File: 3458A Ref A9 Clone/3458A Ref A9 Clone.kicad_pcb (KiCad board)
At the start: 4 copper layers, 50 x 42.5 mm, 44 parts, among them J400 Molex KK 254, J401 Molex KK 254, Q1 MMBF4392, Q401 BD139, U401 ADR/LTZ1000(A), U402 LT1013

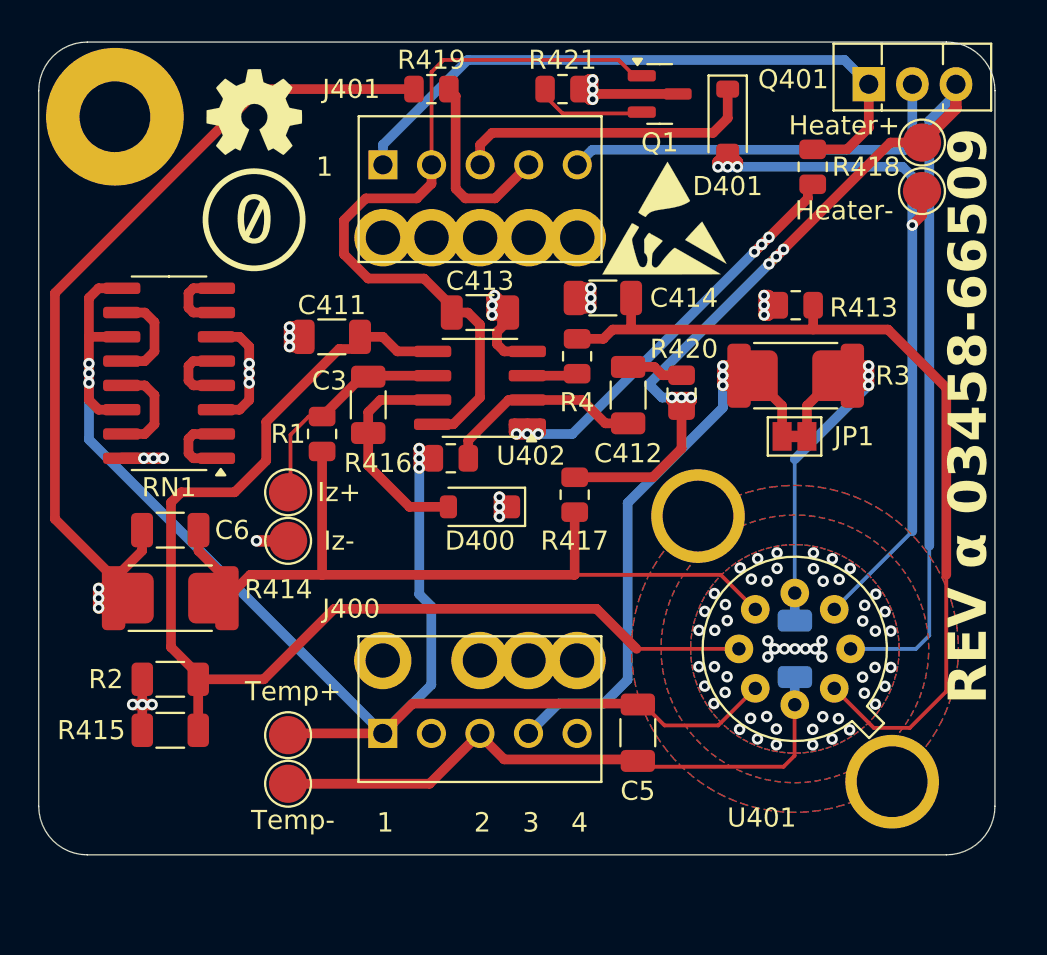
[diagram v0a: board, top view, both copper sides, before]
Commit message: Update to REV β
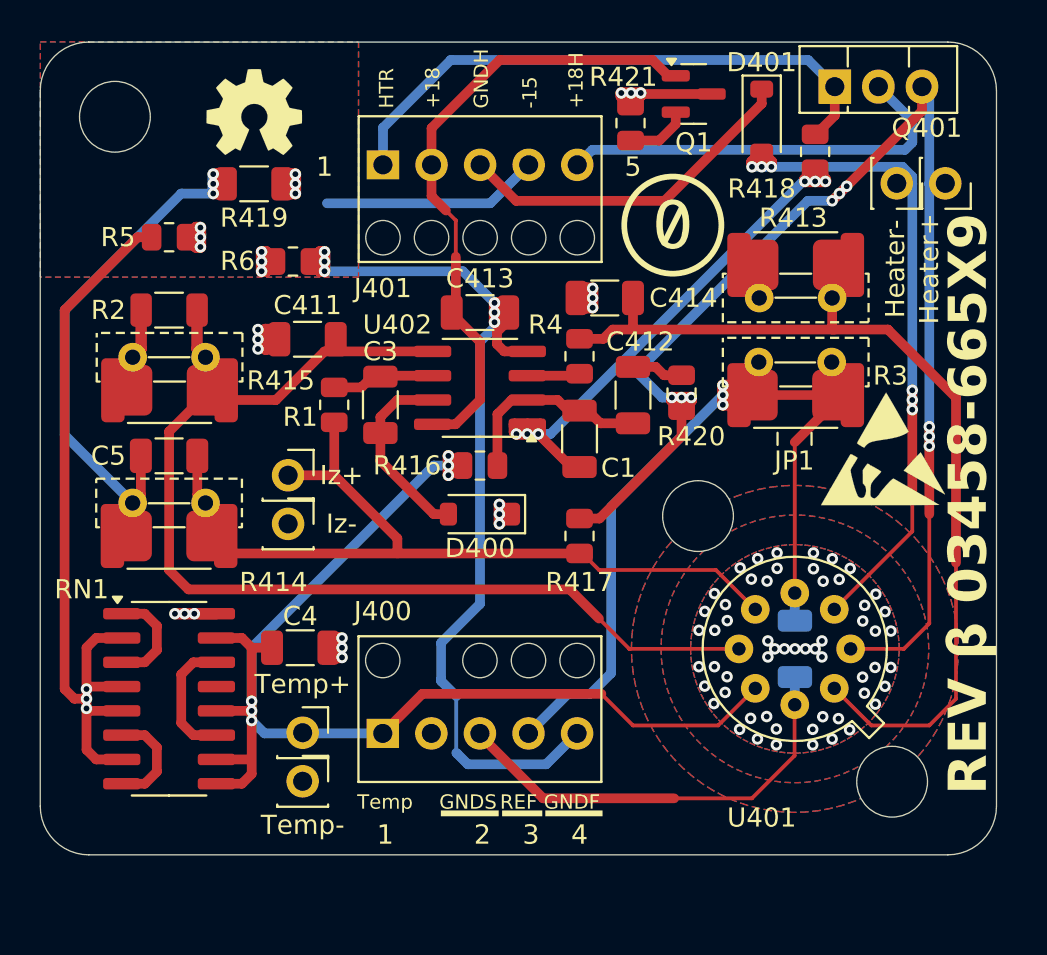
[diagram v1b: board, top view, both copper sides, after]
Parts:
- added C1: 10n, Capacitor_SMD:C_1206_3216Metric, F.Cu at (158.4, 113.5)
- added R5: 19k6, Resistor_SMD:R_0805_2012Metric, F.Cu at (136.9, 103.0)
- added R6: 22k, Resistor_SMD:R_0805_2012Metric, F.Cu at (143.4, 104.3)
- R413: footprint Resistor_SMD:R_0805_2012Metric -> Resistor_SMD:R_1206_3216Metric
- R419: value 1470 -> 1k6; footprint Resistor_SMD:R_0805_2012Metric -> Resistor_SMD:R_1206_3216Metric
- TP1, TP2, TP3, TP4, TP5, TP6: footprint TestPoint:TestPoint_Pad_D2.0mm -> KiCad:PinSocket_1x01_P2.54mm_Vertical
- U401: value ADR/LTZ1000(A) -> ADR1000
- moved R2 19.3 mm to (136.9, 106.8)
- moved C4 18.2 mm to (143.8, 124.5), turned to 0 degrees
- moved R415 17.7 mm to (136.9, 111.0)
- moved RN1 17.0 mm to (136.9, 127.1), turned to 0 degrees
- moved REF** 16.6 mm to (174.2, 114.0)
- moved REF** 14.4 mm to (153.2, 96.1)
- moved R419 10.5 mm to (141.4, 100.2)
- moved REF** 4.28 mm to (176.1, 105.8)
- moved R421 3.98 mm to (161.0, 97.0), turned to 90 degrees
- moved C5 3.89 mm to (136.9, 114.4)
- moved R414 3.25 mm to (136.9, 118.6)
- moved TP5 2.46 mm to (177.5, 100.2), turned to -90 degrees
- moved R417 2.17 mm to (158.4, 118.6)
- moved JP1 2.16 mm to (169.6, 111.3)
- moved R413 2.16 mm to (169.7, 104.4)
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- renumbered C5 to C4, C6 to C5
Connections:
- RN1 pad 10: Net-(RN1E-R5.2) -> J400 (1): Temp
- RN1 pad 11: J400 (1): Temp -> Net-(RN1C-R3.2)
- RN1 pad 12: Net-(RN1E-R5.2) -> J400 (1): Temp
- RN1 pad 13: Net-(RN1B-R2.2) -> unconnected-(RN1D-R4.2-Pad13)
- RN1 pad 14: J400 (1): Temp -> Net-(RN1C-R3.2)
- RN1 pad 15: Net-(RN1B-R2.2) -> J400 (1): Temp
- RN1 pad 2: Net-(RN1A-R1.1) -> J400 (2): REF GND
- RN1 pad 3: J400 (2): REF GND -> Net-(RN1A-R1.1)
- RN1 pad 4: Net-(RN1D-R4.1) -> J400 (2): REF GND
- RN1 pad 5: Net-(RN1D-R4.1) -> J400 (2): REF GND
- RN1 pad 6: J400 (2): REF GND -> Net-(RN1F-R6.1)
- RN1 pad 7: Net-(RN1G-R7.1) -> J400 (2): REF GND
- RN1 pad 8: Net-(RN1G-R7.1) -> Net-(RN1F-R6.1)
- TP3 pad 1: Net-(U402B--) -> ZD-
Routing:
- net J400 (2): REF GND: track 108.4 -> 158.9 mm, vias 16 -> 21
- net J400 (1): Temp: track 82.9 -> 66.0 mm
- net -15: track 10.1 -> 20.8 mm, vias 0 -> 9
- net +7V REF: track 51.0 -> 40.5 mm, vias 18 -> 12
- net Net-(JP1-A): track 22.0 -> 13.8 mm, vias 3 -> 0
- net +18: track 40.6 -> 33.3 mm
- net Net-(RN1C-R3.2): track 0.00 -> 6.75 mm
- net Net-(C1-Pad1): track 25.9 -> 32.4 mm
- net Net-(U402B--): track 11.6 -> 5.40 mm
- net Net-(U402B-+): track 62.0 -> 56.1 mm
- net Net-(RN1F-R6.1): track 0.00 -> 5.48 mm
- net Net-(RN1E-R5.2): track 5.37 -> 0.00 mm
- net Net-(RN1B-R2.2): track 5.37 -> 0.00 mm
- net Net-(RN1G-R7.1): track 3.89 -> 0.00 mm
- net Net-(RN1D-R4.1): track 3.89 -> 0.00 mm
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- added copper zone on B.Cu, net -15
- added copper zone on F.Cu, net -15
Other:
- board text added: "+18"
- board text added: "+18H"
- board text added: "-15"
- board text added: "5"
- board text added: "GNDF"
- board text added: "GNDH"
- board text added: "GNDS"
- board text added: "HTR"
- board text added: "REF"
- board text added: "REV β 03458-665X9"
- board text added: "Temp"
- board text removed: "REV α 03458-66509"
